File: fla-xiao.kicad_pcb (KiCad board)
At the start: 2 copper layers, 50 x 31 mm, 9 parts, among them J1 Conn_PinHeader_1x08_P2.54mm_V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, J2 Conn_PinHeader_1x04_P2.54mm_V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, J3 Conn_PinHeader_2x03_P2.54mm_V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, M1 Module_XIAO-RP2040_SocketSMD, SW1 BUTTON_B3SN

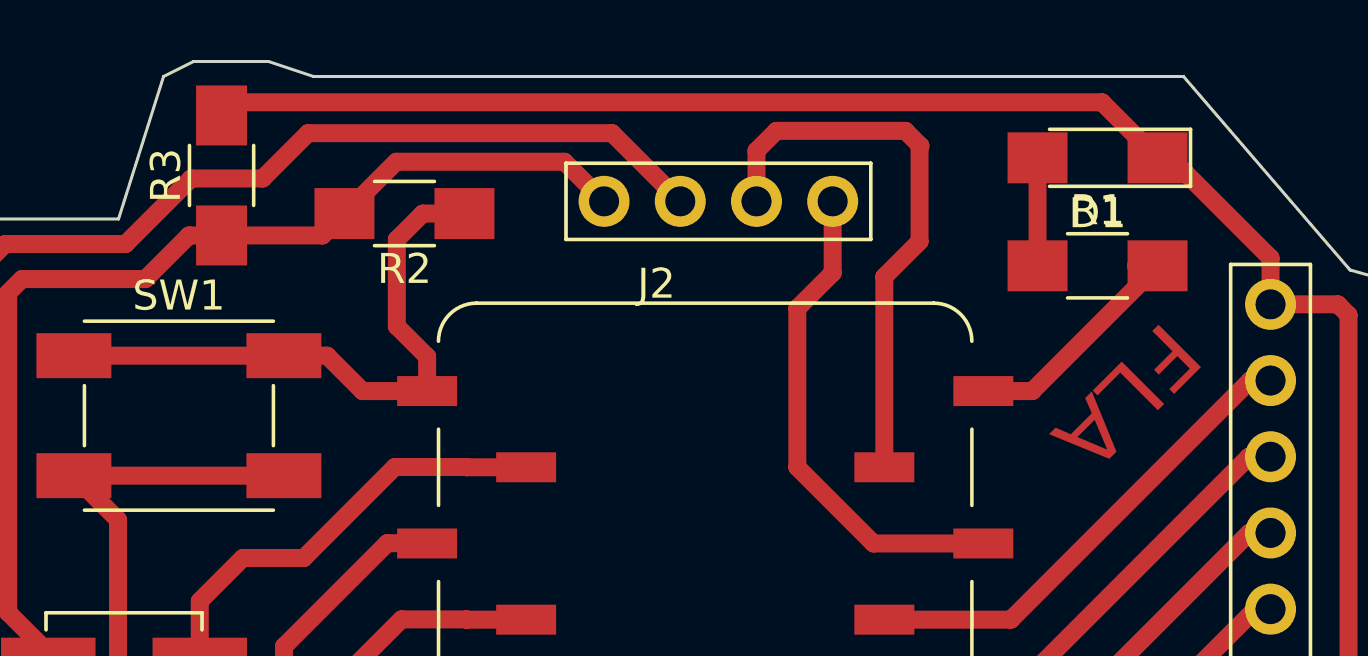
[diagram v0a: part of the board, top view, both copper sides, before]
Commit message: .\fla-xiao.kicad*
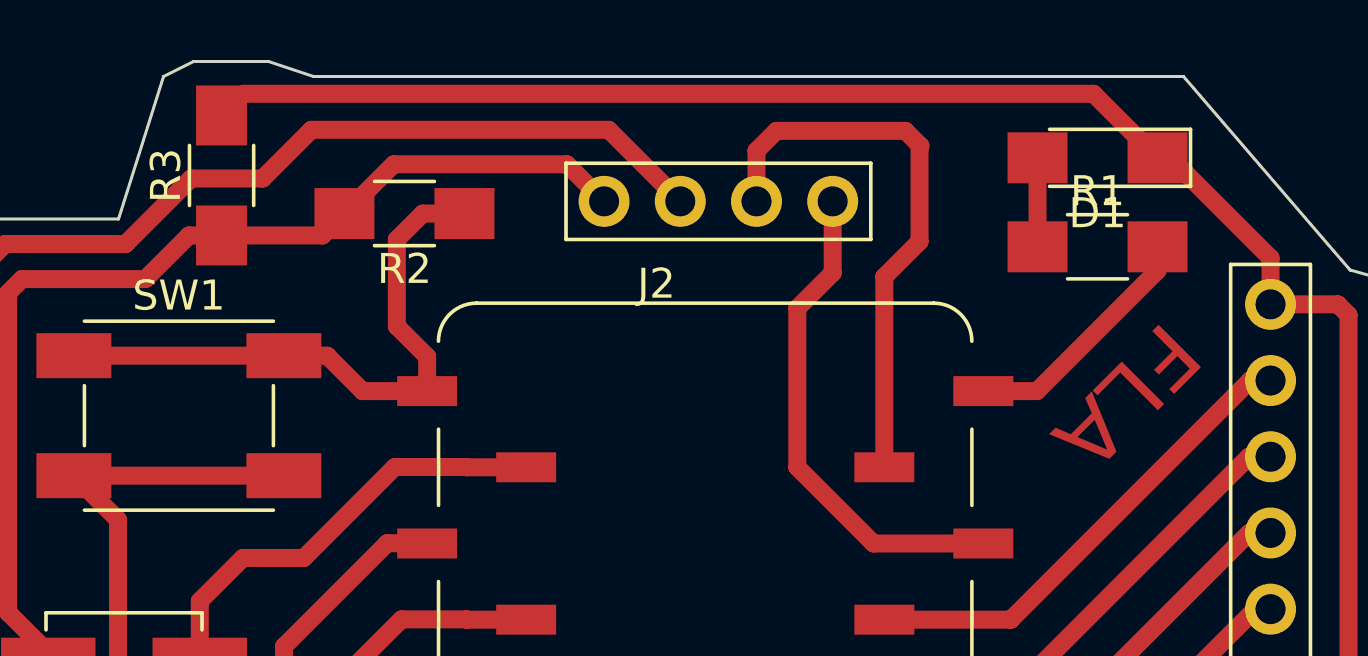
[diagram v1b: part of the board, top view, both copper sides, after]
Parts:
- moved R1 0.63 mm to (161.3, 142.4)
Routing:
- net Net-(D1-A): track 3.60 -> 2.97 mm

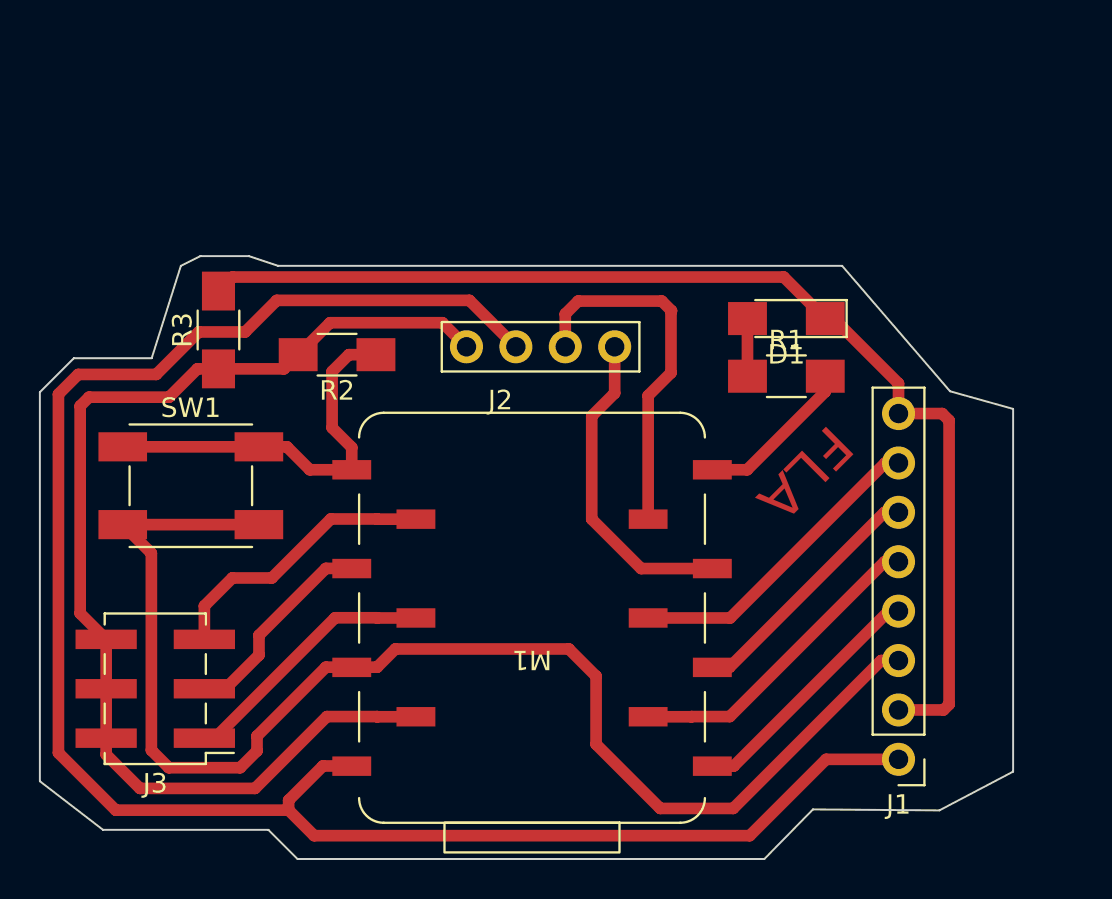
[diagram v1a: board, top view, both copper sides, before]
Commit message: Updated board
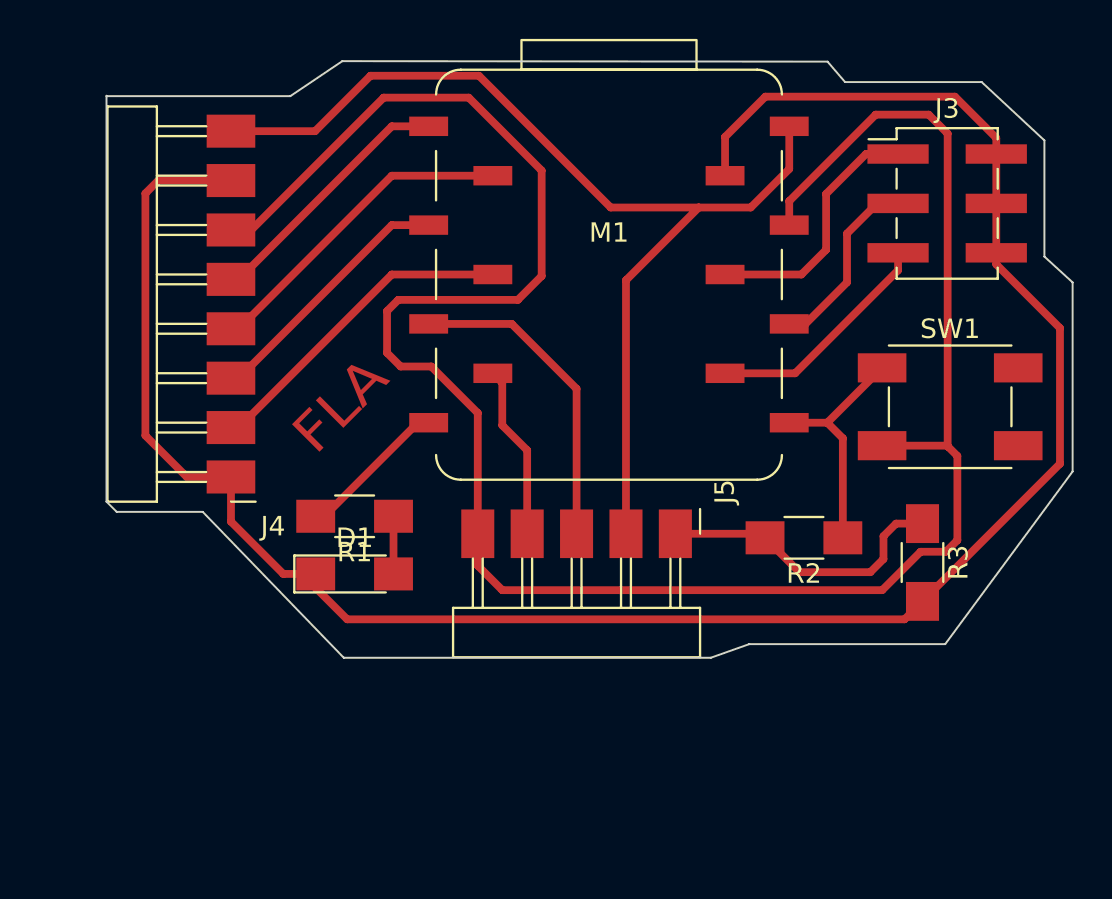
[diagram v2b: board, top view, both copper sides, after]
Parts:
- removed J1: Conn_PinHeader_1x08_P2.54mm_Vertical_THT_D1mm, fab:PinHeader_1x08_P2.54mm_Vertical_THT_D1mm
- removed J2: Conn_PinHeader_1x04_P2.54mm_Vertical_THT_D1mm, fab:PinHeader_1x04_P2.54mm_Vertical_THT_D1mm
- added J4: Conn_PinHeader_1x08_P2.54mm_Horizontal_SMD, fab:PinHeader_1x08_P2.54mm_Horizontal_SMD, F.Cu at (132.7, 147.6)
- added J5: Conn_PinHeader_1x05_P2.54mm_Horizontal_SMD, fab:PinHeader_1x05_P2.54mm_Horizontal_SMD, F.Cu at (155.6, 150.5)
- moved J3 47.8 mm to (169.5, 133.5), turned to 0 degrees
- moved SW1 39.3 mm to (169.7, 144.0)
- moved R3 38.1 mm to (168.3, 152.0), turned to -90 degrees
- moved D1 25.8 mm to (139.1, 152.6), turned to 0 degrees
- moved R2 25.8 mm to (162.2, 150.7)
- moved R1 23.3 mm to (139.1, 149.6), turned to 180 degrees
- moved M1 18.1 mm to (152.1, 137.2), turned to 0 degrees
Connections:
- net +3V3 renamed PWR_3V3
- net Net-(J3-Pin_1) renamed A10
- net Net-(J3-Pin_3) renamed A9
- net Net-(J3-Pin_5) renamed A8
- net Net-(M1-D6) renamed A6
- net Net-(M1-D7) renamed A7
- M1 pad 1: Net-(J1-Pin_4) -> A0
- M1 pad 14: +5V -> PWR_5V
- M1 pad 2: Net-(J1-Pin_5) -> A1
- M1 pad 3: Net-(J1-Pin_6) -> A2
- M1 pad 4: Net-(J1-Pin_7) -> A3
- M1 pad 5: Net-(J2-Pin_1) -> SDA
- M1 pad 6: Net-(J2-Pin_2) -> SCL
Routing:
- net +5V: track 96.0 -> 0.00 mm
- net PWR_5V: track 0.00 -> 54.0 mm
- net PWR_3V3: track 69.6 -> 113.3 mm
- net Net-(J2-Pin_2): track 18.8 -> 0.00 mm
- net A1: track 0.00 -> 16.7 mm
- net A3: track 0.00 -> 16.7 mm
- net Net-(J2-Pin_1): track 16.6 -> 0.00 mm
- net SDA: track 0.00 -> 16.4 mm
- net Net-(J1-Pin_5): track 16.2 -> 0.00 mm
- net Net-(J1-Pin_7): track 16.2 -> 0.00 mm
- net Net-(J1-Pin_6): track 13.6 -> 0.00 mm
- net A0: track 0.00 -> 13.4 mm
- net A2: track 0.00 -> 13.4 mm
- net Net-(J1-Pin_4): track 12.9 -> 0.00 mm
- net SCL: track 0.00 -> 8.98 mm
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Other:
- board size 50 x 31 mm -> 49.7 x 30.7 mm
